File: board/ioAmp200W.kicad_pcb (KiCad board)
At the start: 2 copper layers, 1.4 x 9.2 mm, 33 parts, among them J1 USB4105-GF-A-120, J2 USB4105-GF-A-120, J4 SM03B-SRSS-TB, U1 RP2350_60QFN, U2 TPS26750SRSMR, U3 TPD4S480RUKR, U4 ADAU1761BCPZ-RL, Y1 ABM8-272-T3

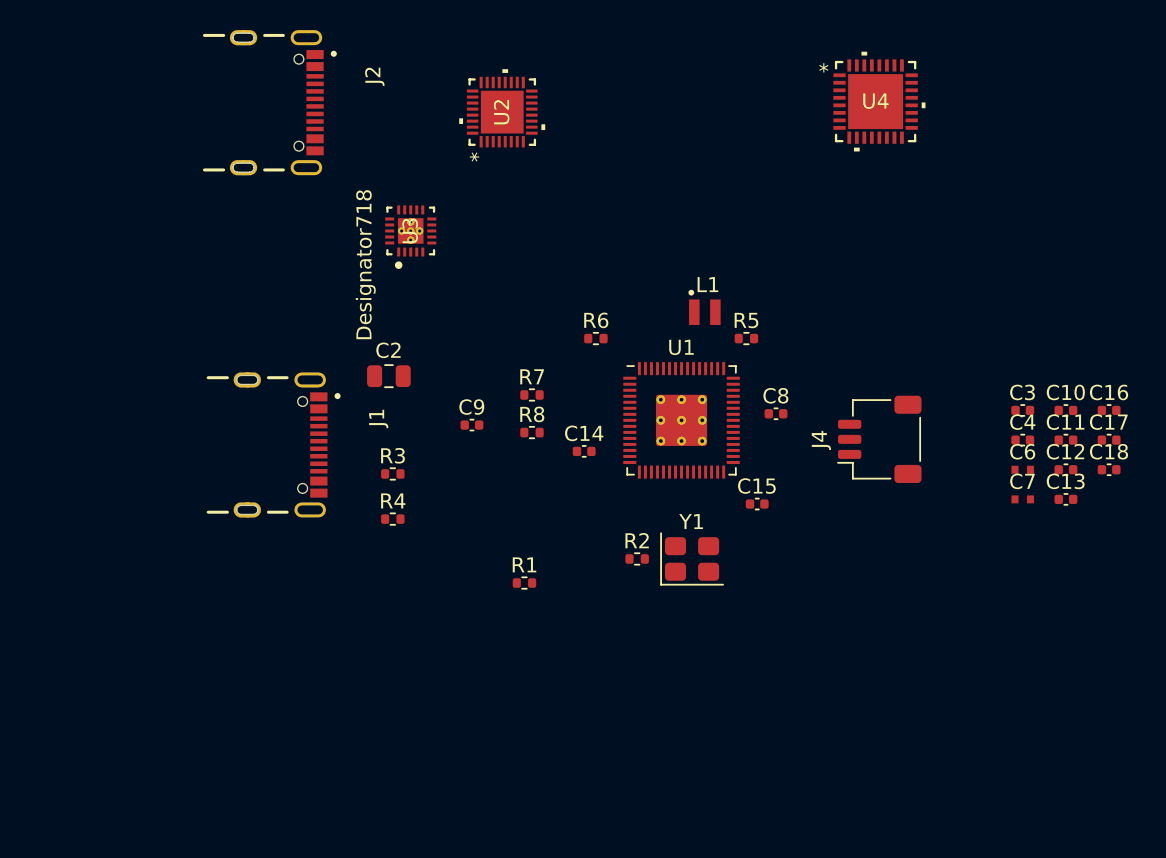
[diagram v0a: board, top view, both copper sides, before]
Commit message: work
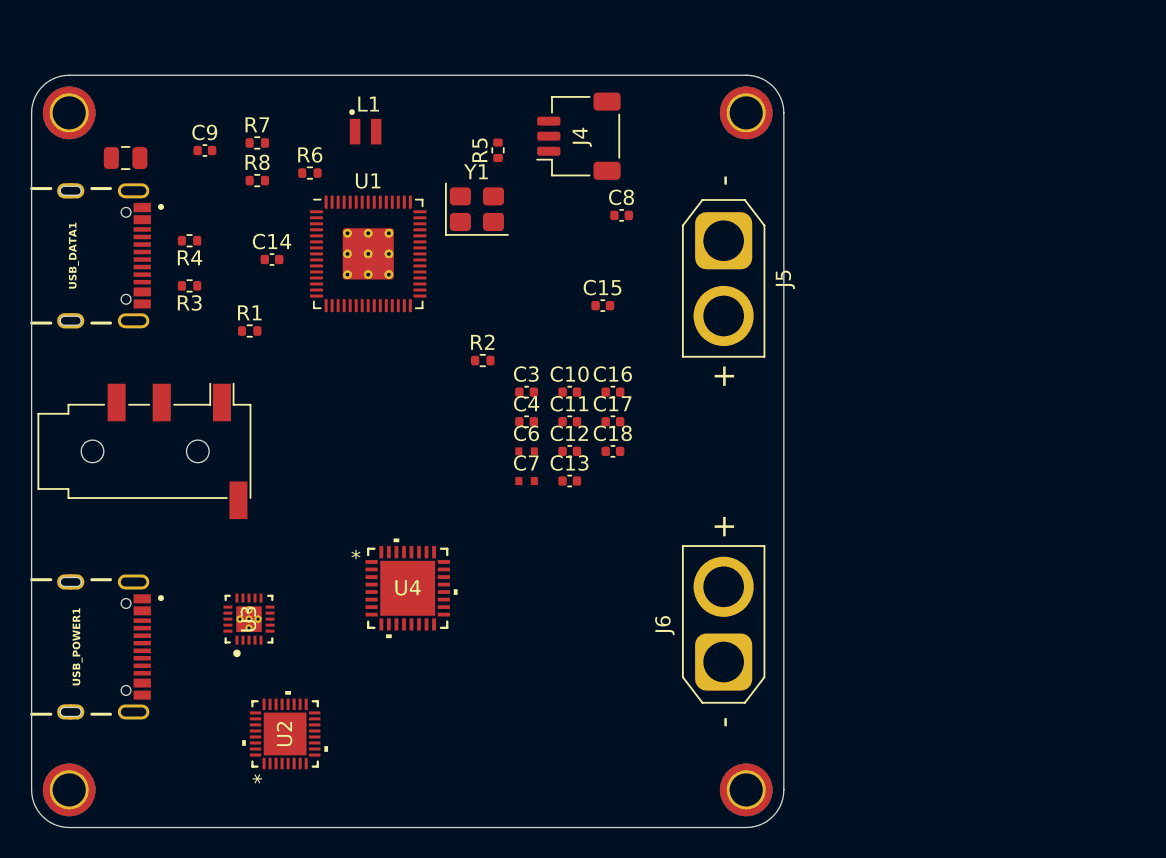
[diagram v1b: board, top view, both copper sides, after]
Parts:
- added H1: MountingHole_Pad_MP, MountingHole:MountingHole_2.2mm_M2_ISO7380_Pad_TopBottom, F.Cu at (102.5, 102.5)
- added H2: MountingHole_Pad_MP, MountingHole:MountingHole_2.2mm_M2_ISO7380_Pad_TopBottom, F.Cu at (147.5, 102.5)
- added H3: MountingHole_Pad_MP, MountingHole:MountingHole_2.2mm_M2_ISO7380_Pad_TopBottom, F.Cu at (147.5, 147.5)
- added H4: MountingHole_Pad_MP, MountingHole:MountingHole_2.2mm_M2_ISO7380_Pad_TopBottom, F.Cu at (102.5, 147.5)
- added J3: AudioJack3_Ground, Connector_Audio:Jack_3.5mm_PJ320D_Horizontal, F.Cu at (108.8, 125.0)
- added J5: Conn_01x02_Socket, Connector_AMASS:AMASS_XT30U-F_1x02_P5.0mm_Vertical, F.Cu at (146.0, 111.0)
- added J6: Conn_01x02_Socket, Connector_AMASS:AMASS_XT30U-F_1x02_P5.0mm_Vertical, F.Cu at (146.0, 139.0)
- moved U4 44.9 mm to (125.0, 134.1)
- moved U2 43.8 mm to (116.8, 143.8)
- moved USB_POWER1 38.0 mm to (102.6, 138.0)
- moved C16 33.0 mm to (138.6, 121.1)
- moved C17 33.0 mm to (138.6, 123.0)
- moved C18 33.0 mm to (138.6, 125.0)
- moved C10 33.0 mm to (135.8, 121.1)
- moved C11 33.0 mm to (135.8, 123.0)
- moved C12 33.0 mm to (135.8, 125.0)
- moved C13 33.0 mm to (135.8, 127.0)
- moved C3 33.0 mm to (132.9, 121.1)
- moved C4 33.0 mm to (132.9, 123.0)
- moved C6 33.0 mm to (132.9, 125.0)
- moved C7 33.0 mm to (132.9, 127.0)
- moved J4 28.4 mm to (136.4, 104.0)
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- renumbered J1 to USB_DATA1, J2 to USB_POWER1
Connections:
- USB_POWER1 pad A1_B12: unconnected-(J2-GND-PadA1_B12) -> GND
- USB_POWER1 pad B1_A12: unconnected-(J2-GND__1-PadB1_A12) -> GND
- USB_POWER1 pad SH1: unconnected-(J2-SHELL_GND-PadSH1) -> GND
- USB_POWER1 pad SH2: unconnected-(J2-SHELL_GND__1-PadSH2) -> GND
- USB_POWER1 pad SH3: unconnected-(J2-SHELL_GND__2-PadSH3) -> GND
- USB_POWER1 pad SH4: unconnected-(J2-SHELL_GND__3-PadSH4) -> GND
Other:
- board size 1.4 x 9.2 mm -> 50 x 50 mm
